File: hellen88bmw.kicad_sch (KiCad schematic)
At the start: 305 parts, among them J1 920-462A2021Y10101, J14 VRIN1, J15 VRIN2, J16 VROUT1, J17 XH-8A, J18 PJ-3250-5A, J19 MiniFit, J2 DNP, J20 ETB, J21 ETB, J3 Conn_01x06, J4 Conn_01x05, J5 Conn_01x12, J6 Conn_01x12, J7 Conn_01x12, J8 Conn_01x12, J9 Conn_01x12, M1 Module-power12-0.2, M10 Module-ign8-0.1, M11 Module-mcu144-0.5, M12 Module-knock-0.1, M13 Module-sd-0.1, M2 Module-can-0.1, M3 Module-wbo-0.2, M4 Module-can-0.1, M5 Module-power5-0.2, M6 Module-vr-0.1, M7 Module-input-0.1, M8 Module-knock-0.1, M9 Module-output-0.2, P1 P, P15 Pad, P16 Pad, P17 Pad, P18 Pad, P19 Pad, P2 P, P21 Pad, P22 Pad, P23 Pad, P24 Pad, P25 Pad, P26 Pad, P27 Pad, P28 Pad, P29 Pad, P3 P, P30 Pad, P31 Pad, P32 Pad, P4 P, P5 P, P6 P, Q1 NGD8201AN, Q10 AUIPS2041L, Q2 NGD8201AN, Q3 NGD8201AN, Q4 NGD8201AN, Q5 NGD8201AN, Q6 NGD8201AN, Q7 NGD8201AN, Q8 NGD8201AN, Q9 AUIPS2041L, SW1 RESET, SW2 RESET, U1 MPXA6115A, U2 MPX4_MAP, U3 LIS2DW12TR, U4 LPS25HB, U5 MCP6002-xSN, U6 L6205PD

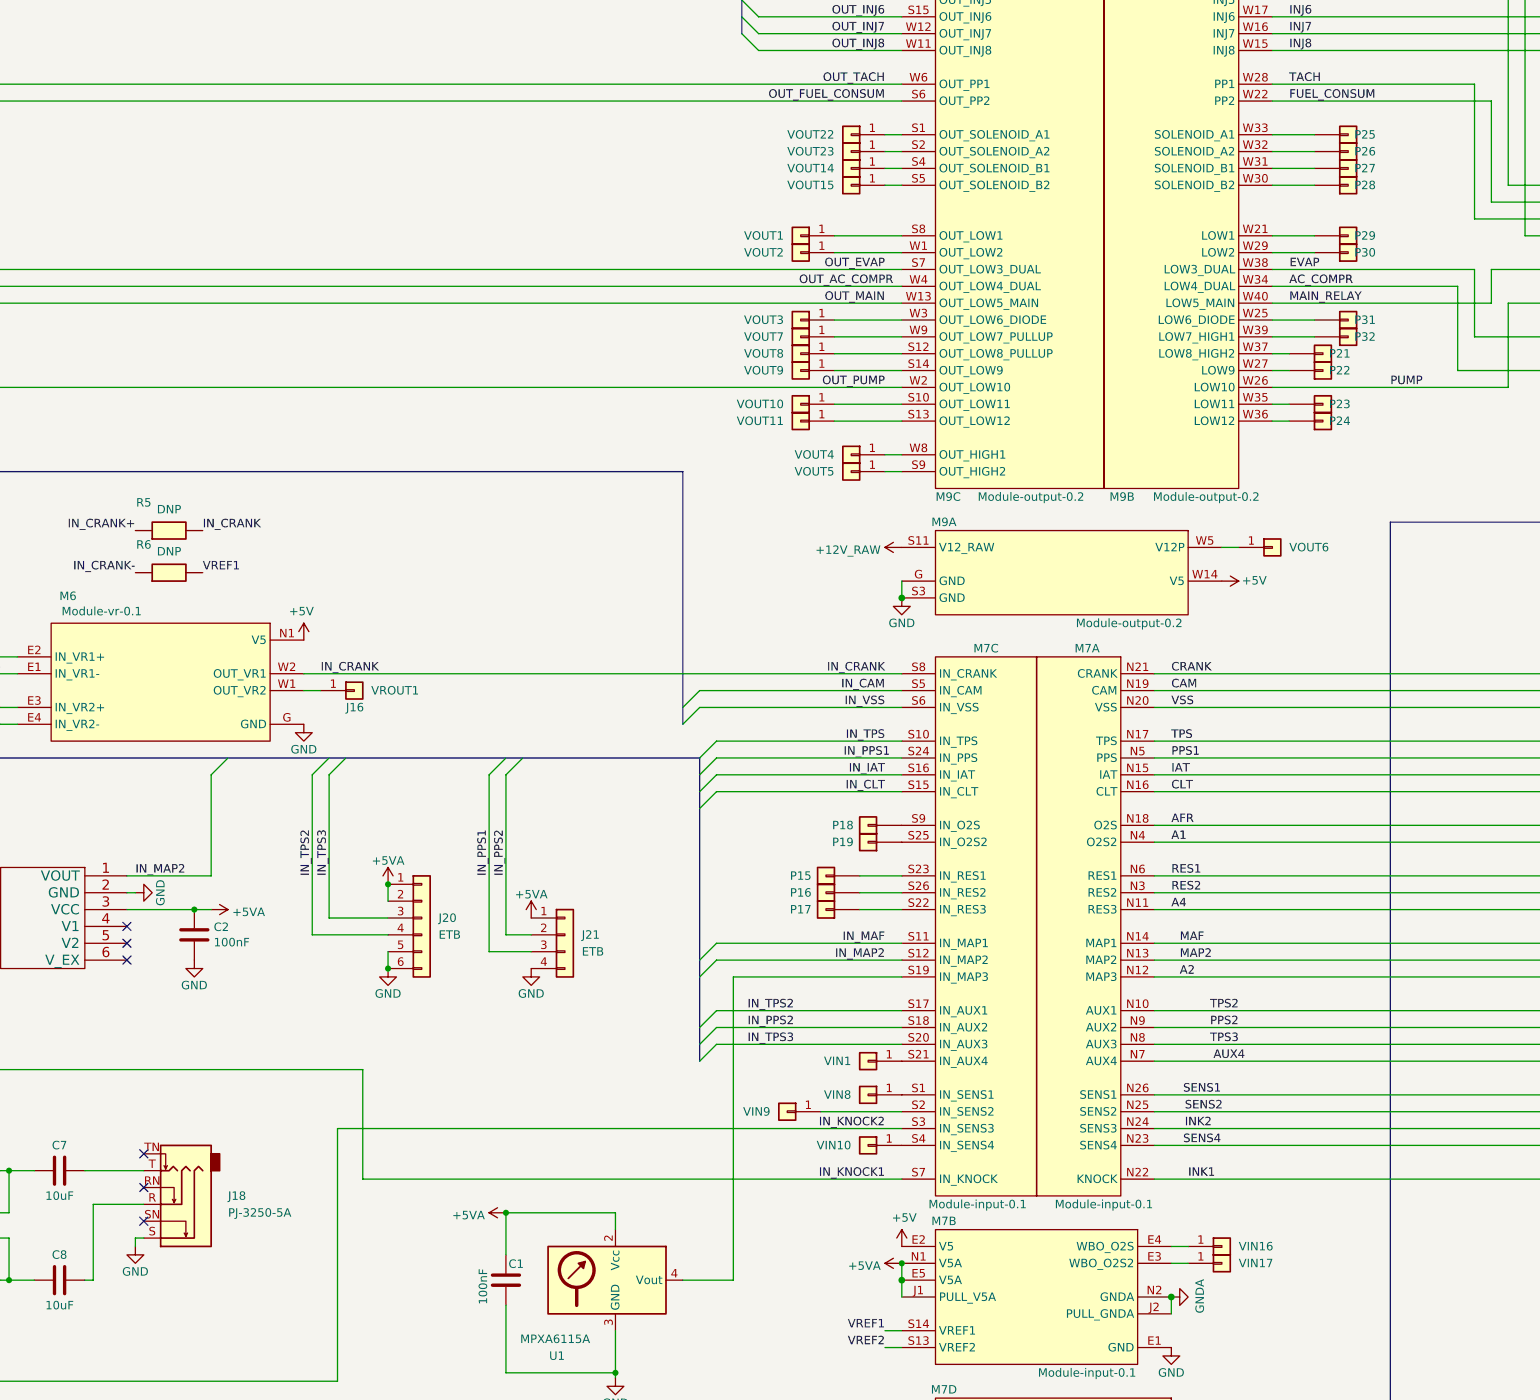
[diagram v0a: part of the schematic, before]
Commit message: PCB refactoring started
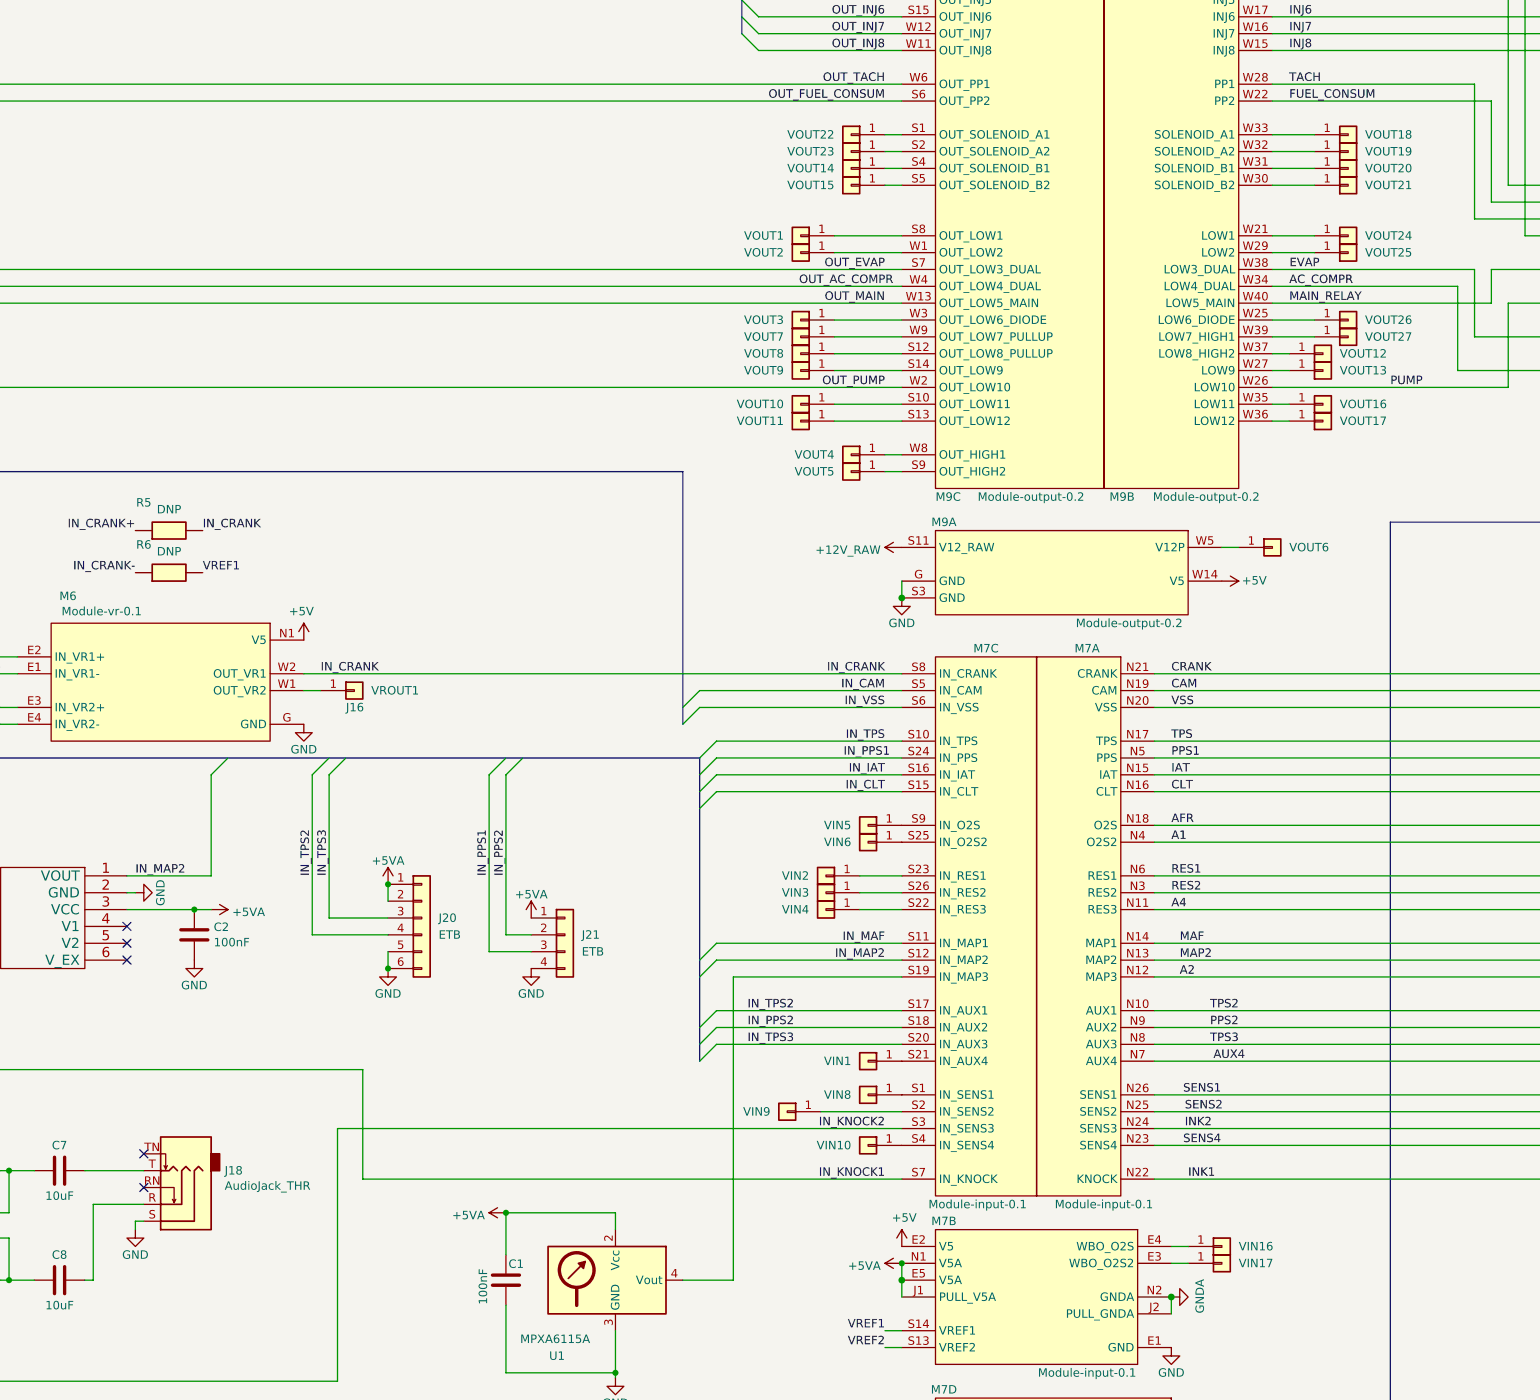
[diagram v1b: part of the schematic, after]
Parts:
- removed J18: PJ-3250-5A, Connector_Audio:Jack_3.5mm_CUI_SJ1-3535NG_Horizontal, symbol Connector:AudioJack3_Switch
- removed P15, P16, P17, P18, P19, P21, P22, P23, P24, P25, P26, P27, P28, P29, P30, P31, P32: Pad, hellen-one-common:PAD-TH, symbol hellen-one-common:Pad
- added J18: AudioJack_THR, hellen-one-common:Jack_3.5mm_PJ-3250-5A, symbol hellen-one-common:AudioJack_THR
- added VIN2, VIN3, VIN4, VIN5, VIN6: VIN8, Connector_PinHeader_1.00mm:PinHeader_1x01_P1.00mm_Vertical, symbol Connector_Generic:Conn_01x01
- added VOUT12, VOUT13, VOUT16, VOUT17, VOUT18, VOUT19, VOUT20, VOUT21, VOUT24, VOUT25, VOUT26, VOUT27: VOUT4, Connector_PinHeader_1.00mm:PinHeader_1x01_P1.00mm_Vertical, symbol Connector_Generic:Conn_01x01
- G1, G4: footprint footprints:LOGO -> hellen-one-common:LOGO
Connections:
- net GND: now also J18.S
- net at M9.W35 (LOW11): now also VOUT16.1 (Pin_1)
- net at M7.S22 (IN_RES3): now also VIN4.1 (Pin_1)
- net at M9.W21 (LOW1): now also VOUT24.1 (Pin_1)
- net at M9.W37 (LOW8_HIGH2): now also VOUT12.1 (Pin_1)
- net at M9.W25 (LOW6_DIODE): now also VOUT26.1 (Pin_1)
- net at M7.S23 (IN_RES1): now also VIN2.1 (Pin_1)
- net at M7.S25 (IN_O2S2): now also VIN6.1 (Pin_1)
- net at M7.S26 (IN_RES2): now also VIN3.1 (Pin_1)
- net at M7.S9 (IN_O2S): now also VIN5.1 (Pin_1)
- net at M9.W33 (SOLENOID_A1): now also VOUT18.1 (Pin_1)
- net at C8.2: now also J18.R
- net at C7.2: now also J18.T
- net at M9.W29 (LOW2): now also VOUT25.1 (Pin_1)
- net at M9.W39 (LOW7_HIGH1): now also VOUT27.1 (Pin_1)
- net at M9.W27 (LOW9): now also VOUT13.1 (Pin_1)
- net at M9.W30 (SOLENOID_B2): now also VOUT21.1 (Pin_1)
- net at M9.W31 (SOLENOID_B1): now also VOUT20.1 (Pin_1)
- net at M9.W32 (SOLENOID_A2): now also VOUT19.1 (Pin_1)
- net at M9.W36 (LOW12): now also VOUT17.1 (Pin_1)
- no-connect marks 105 -> 104
